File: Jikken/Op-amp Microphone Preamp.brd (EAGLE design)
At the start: 100 x 80 mm, 11 parts, among them IC1 AD822N

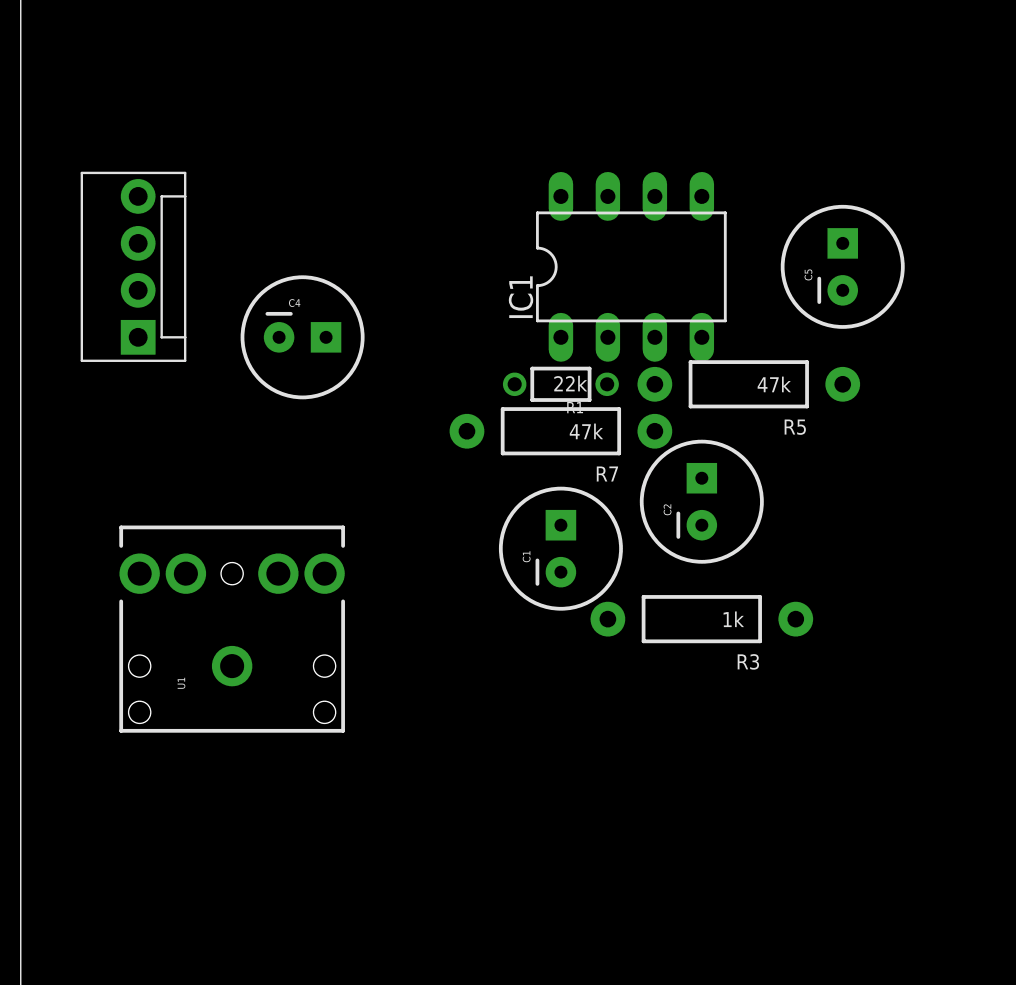
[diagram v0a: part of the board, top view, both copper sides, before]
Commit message: Preamp
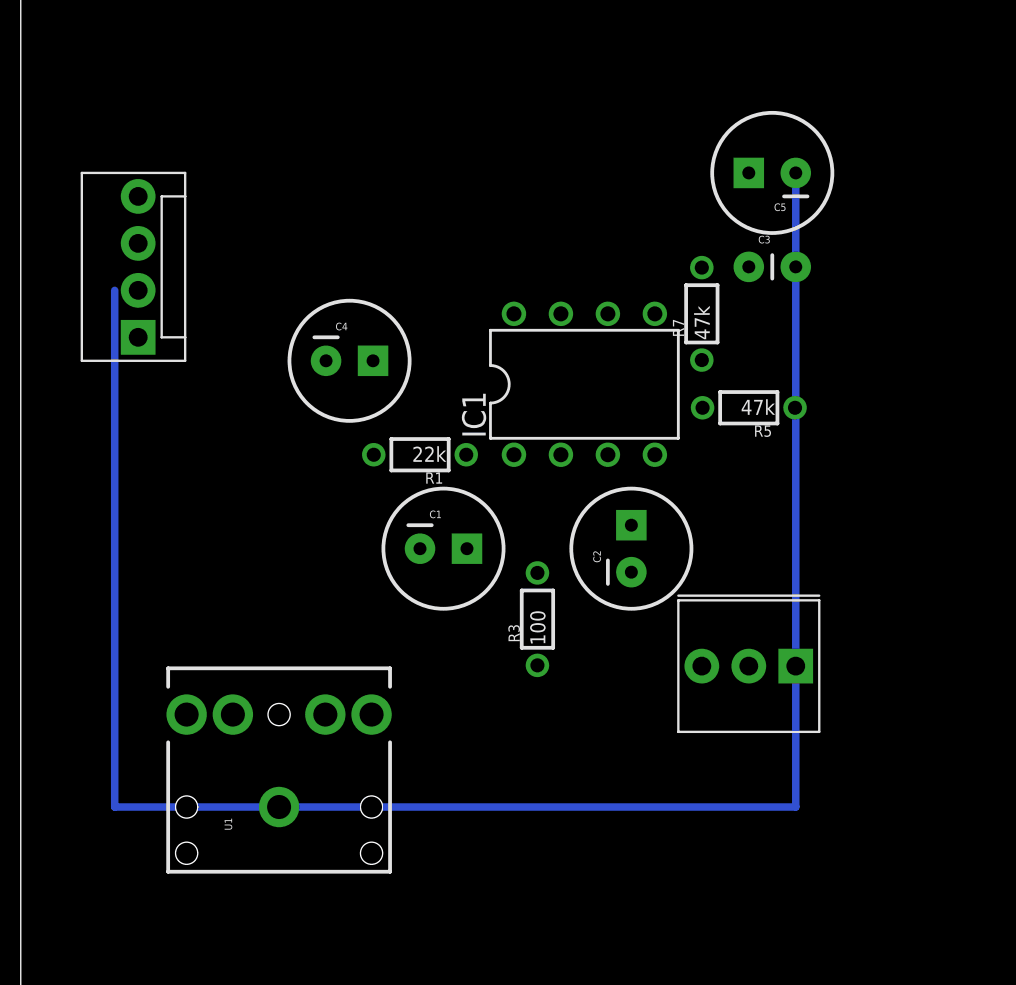
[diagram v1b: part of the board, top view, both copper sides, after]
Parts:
- added C3: 0.1uF, SparkFun:CAP-PTH-SMALL
- added TRIMPOT: 10k, My Library:3362U
- IC1: value AD822N -> LF356N; device analog-devices:DIL08 -> My Library:DIL08
- R3: value 1k -> 100; device SparkFun:AXIAL-0.4 -> SparkFun:1/6W-RES
- R5, R7: device SparkFun:AXIAL-0.4 -> SparkFun:1/6W-RES
- moved R7 9.92 mm to (36.8, 47.0), turned to 90 degrees
- moved R3 8.89 mm to (27.9, 30.5), turned to 90 degrees
- moved R1 8.52 mm to (21.6, 39.4)
- moved U1 8.03 mm to (14.0, 20.3)
- moved IC1 6.84 mm to (30.5, 43.2)
- moved C1 6.35 mm to (22.9, 34.3), turned to 0 degrees
- moved C5 6.35 mm to (40.6, 54.6), turned to 180 degrees
- moved C2 4.58 mm to (33.0, 34.3)
- moved C4 2.84 mm to (17.8, 44.5)
- moved R5 1.27 mm to (39.4, 41.9)
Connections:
- new net N$4: R3.1, TRIMPOT.P$2, TRIMPOT.P$3
- net GND: now also C3.2, R5.1, TRIMPOT.P$1; no longer R3.P$1, R5.P$1
- net N$2: now also R3.2; no longer R3.P$2
- net N$3: now also IC1.6; no longer IC1.1
- net N$6: now also R5.2, R7.1; no longer R5.P$2, R7.P$1
- net VCC: now also C3.1, IC1.7, R7.2; no longer IC1.8, R7.P$2
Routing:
- net GND: track 0.00 -> 99.1 mm
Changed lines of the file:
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@@
 </autorouter>
 <elements>
-<element name="IC1" library="analog-devices" package="DIL08" value="AD822N" x="33.02" y="49.53">
-<attribute name="OC_NEWARK" value="unknown" x="52.07" y="17.78" size="1.778" layer="27" display="off"/>
-<attribute name="MPN" value="" x="52.07" y="17.78" size="1.778" layer="27" display="off"/>
-<attribute name="MF" value="" x="52.07" y="17.78" size="1.778" layer="27" display="off"/>
-<attribute name="OC_FARNELL" value="1438581" x="52.07" y="17.78" size="1.778" layer="27" display="off"/>
-</element>
-<element name="R1" library="My Library" package="1/6W-RES" value="22k" x="29.21" y="43.18" rot="R180"/>
-<element name="R3" library="SparkFun" package="AXIAL-0.4" value="1k" x="36.83" y="30.48" rot="R180"/>
-<element name="C1" library="SparkFun" package="CPOL-RADIAL-100UF-25V" value="10u" x="29.21" y="34.29" rot="R90"/>
-<element name="R5" library="SparkFun" package="AXIAL-0.4" value="47k" x="39.37" y="43.18" rot="R180"/>
-<element name="U1" library="SparkFun" package="AUDIO-JACK" value="" x="11.43" y="27.94" rot="R90"/>
-<element name="R7" library="SparkFun" package="AXIAL-0.4" value="47k" x="29.21" y="40.64" rot="R180"/>
-<element name="C5" library="SparkFun" package="CPOL-RADIAL-100UF-25V" value="100u" x="44.45" y="49.53" rot="R90"/>
+<element name="R1" library="My Library" package="1/6W-RES" value="22k" x="21.59" y="39.37" rot="R180"/>
+<element name="R3" library="SparkFun" package="1/6W-RES" value="100" x="27.94" y="30.48" rot="R90"/>
+<element name="C1" library="SparkFun" package="CPOL-RADIAL-100UF-25V" value="10u" x="22.86" y="34.29"/>
+<element name="R5" library="SparkFun" package="1/6W-RES" value="47k" x="39.37" y="41.91" rot="R180"/>
+<element name="U1" library="SparkFun" package="AUDIO-JACK" value="" x="13.97" y="20.32" rot="R90"/>
+<element name="R7" library="SparkFun" package="1/6W-RES" value="47k" x="36.83" y="46.99" rot="R90"/>
+<element name="C5" library="SparkFun" package="CPOL-RADIAL-100UF-25V" value="100u" x="40.64" y="54.61" rot="R180"/>
 <element name="JP2" library="SparkFun" package="MOLEX-1X4" value="" x="6.35" y="45.72" rot="R90"/>
-<element name="C4" library="SparkFun" package="CPOL-RADIAL-100UF-25V" value="10u" x="15.24" y="45.72"/>
-<element name="C2" library="SparkFun" package="CPOL-RADIAL-100UF-25V" value="10u" x="36.83" y="36.83" rot="R90"/>
+<element name="C4" library="SparkFun" package="CPOL-RADIAL-100UF-25V" value="10u" x="17.78" y="44.45"/>
+<element name="C2" library="SparkFun" package="CPOL-RADIAL-100UF-25V" value="10u" x="33.02" y="34.29" rot="R90"/>
+<element name="IC1" library="My Library" package="DIL08" value="LF356N" x="30.48" y="43.18"/>
+<element name="TRIMPOT" library="My Library" package="3362U" value="10k" x="41.91" y="30.48" rot="R180"/>
+<element name="C3" library="SparkFun" package="CAP-PTH-SMALL" value="0.1uF" x="39.37" y="49.53"/>
 </elements>
 <signals>
 <signal name="N$3">
 <contactref element="R1" pad="2"/>
-<contactref element="IC1" pad="1"/>
 <contactref element="C4" pad="1"/>
-<wire x1="26.71" y1="43.18" x2="29.21" y2="45.72" width="0" layer="19" extent="1-1"/>
-<wire x1="16.51" y1="45.72" x2="29.21" y2="45.72" width="0" layer="19" extent="1-1"/>
+<contactref element="IC1" pad="6"/>
+<wire x1="19.05" y1="44.45" x2="31.75" y2="46.99" width="0" layer="19" extent="1-1"/>
+<wire x1="19.09" y1="39.37" x2="19.05" y2="44.45" width="0" layer="19" extent="1-1"/>
 </signal>
 <signal name="N$5">
-<contactref element="IC1" pad="2"/>
 <contactref element="C1" pad="1"/>
 <contactref element="R1" pad="1"/>
-<wire x1="31.71" y1="43.18" x2="31.75" y2="45.72" width="0" layer="19" extent="1-1"/>
-<wire x1="29.21" y1="35.56" x2="31.71" y2="43.18" width="0" layer="19" extent="1-1"/>
+<contactref element="IC1" pad="2"/>
+<wire x1="24.13" y1="34.29" x2="24.09" y2="39.37" width="0" layer="19" extent="1-1"/>
+<wire x1="29.21" y1="39.37" x2="24.13" y2="34.29" width="0" layer="19" extent="1-1"/>
 </signal>
 <signal name="N$2">
-<contactref element="R3" pad="P$2"/>
+<contactref element="R3" pad="2"/>
 <contactref element="C1" pad="2"/>
-<wire x1="29.21" y1="33.02" x2="31.75" y2="30.48" width="0" layer="19" extent="1-1"/>
+<wire x1="21.59" y1="34.29" x2="27.94" y2="32.98" width="0" layer="19" extent="1-1"/>
 </signal>
 <signal name="GND">
+<contactref element="C5" pad="2"/>
+<contactref element="JP2" pad="2"/>
 <contactref element="IC1" pad="4"/>
-<contactref element="C5" pad="2"/>
-<contactref element="R5" pad="P$1"/>
+<contactref element="R5" pad="1"/>
 <contactref element="U1" pad="SLEEVE"/>
-<contactref element="JP2" pad="2"/>
-<contactref element="R3" pad="P$1"/>
-<wire x1="44.45" y1="43.18" x2="44.45" y2="48.26" width="0" layer="19" extent="1-1"/>
-<wire x1="36.83" y1="45.72" x2="44.45" y2="48.26" width="0" layer="19" extent="1-1"/>
-<wire x1="41.91" y1="30.48" x2="44.45" y2="43.18" width="0" layer="19" extent="1-1"/>
-<wire x1="6.35" y1="48.26" x2="36.83" y2="45.72" width="0" layer="19" extent="1-1"/>
-<wire x1="11.43" y1="27.94" x2="6.35" y2="48.26" width="0" layer="19" extent="1-1"/>
+<contactref element="TRIMPOT" pad="P$1"/>
+<contactref element="C3" pad="2"/>
+<wire x1="41.91" y1="54.61" x2="41.91" y2="20.32" width="0.4064" layer="16"/>
+<wire x1="41.91" y1="20.32" x2="5.08" y2="20.32" width="0.4064" layer="16"/>
+<wire x1="5.08" y1="20.32" x2="5.08" y2="48.26" width="0.4064" layer="16"/>
+<wire x1="41.91" y1="54.61" x2="41.91" y2="49.53" width="0" layer="19" extent="1-1"/>
+<wire x1="6.35" y1="48.26" x2="5.08" y2="48.26" width="0" layer="19" extent="16-16"/>
+<wire x1="41.87" y1="41.91" x2="41.91" y2="49.53" width="0" layer="19" extent="1-1"/>
+<wire x1="41.91" y1="27.94" x2="41.91" y2="20.32" width="0" layer="19" extent="16-16"/>
+<wire x1="34.29" y1="39.37" x2="41.87" y2="41.91" width="0" layer="19" extent="1-1"/>
+<wire x1="13.97" y1="20.32" x2="5.08" y2="20.32" width="0" layer="19" extent="16-16"/>
 </signal>
 <signal name="N$6">
-<contactref element="R5" pad="P$2"/>
-<contactref element="R7" pad="P$1"/>
+<contactref element="R5" pad="2"/>
+<contactref element="R7" pad="1"/>
+<contactref element="C2" pad="1"/>
 <contactref element="IC1" pad="3"/>
-<contactref element="C2" pad="1"/>
-<wire x1="34.29" y1="40.64" x2="34.29" y2="45.72" width="0" layer="19" extent="1-1"/>
-<wire x1="34.29" y1="40.64" x2="34.29" y2="40.64" width="0" layer="19" extent="1-1"/>
-<wire x1="36.83" y1="38.1" x2="34.29" y2="40.64" width="0" layer="19" extent="1-1"/>
+<wire x1="36.87" y1="41.91" x2="36.83" y2="44.49" width="0" layer="19" extent="1-1"/>
+<wire x1="31.75" y1="39.37" x2="36.87" y2="41.91" width="0" layer="19" extent="1-1"/>
+<wire x1="33.02" y1="35.56" x2="31.75" y2="39.37" width="0" layer="19" extent="1-1"/>
 </signal>
 <signal name="VCC">
-<contactref element="IC1" pad="8"/>
 <contactref element="JP2" pad="3"/>
-<contactref element="R7" pad="P$2"/>
+<contactref element="R7" pad="2"/>
 <contactref element="C5" pad="1"/>
-<wire x1="29.21" y1="53.34" x2="44.45" y2="50.8" width="0" layer="19" extent="1-1"/>
-<wire x1="24.13" y1="40.64" x2="29.21" y2="53.34" width="0" layer="19" extent="1-1"/>
-<wire x1="6.35" y1="50.8" x2="24.13" y2="40.64" width="0" layer="19" extent="1-1"/>
+<contactref element="IC1" pad="7"/>
+<contactref element="C3" pad="1"/>
+<wire x1="39.37" y1="49.53" x2="39.37" y2="54.61" width="0" layer="19" extent="1-1"/>
+<wire x1="36.83" y1="49.49" x2="39.37" y2="49.53" width="0" layer="19" extent="1-1"/>
+<wire x1="29.21" y1="46.99" x2="36.83" y2="49.49" width="0" layer="19" extent="1-1"/>
+<wire x1="6.35" y1="50.8" x2="29.21" y2="46.99" width="0" layer="19" extent="1-1"/>
 </signal>
 <signal name="N$13">
 <contactref element="C4" pad="2"/>
 <contactref element="JP2" pad="1"/>
-<wire x1="6.35" y1="45.72" x2="13.97" y2="45.72" width="0" layer="19" extent="1-1"/>
+<wire x1="6.35" y1="45.72" x2="16.51" y2="44.45" width="0" layer="19" extent="1-1"/>
 </signal>
 <signal name="N$8">
 <contactref element="C2" pad="2"/>
 <contactref element="U1" pad="TIP"/>
-<wire x1="16.43" y1="32.94" x2="36.83" y2="35.56" width="0" layer="19" extent="1-1"/>
+<wire x1="18.97" y1="25.32" x2="33.02" y2="33.02" width="0" layer="19" extent="1-1"/>
 </signal>
 <signal name="N$9">
 <contactref element="U1" pad="RING"/>
 </signal>
+<signal name="N$4">
+<contactref element="R3" pad="1"/>
+<contactref element="TRIMPOT" pad="P$2"/>
+<contactref element="TRIMPOT" pad="P$3"/>
+<wire x1="36.83" y1="27.94" x2="27.94" y2="27.98" width="0" layer="19" extent="1-1"/>
+<wire x1="39.37" y1="27.94" x2="36.83" y2="27.94" width="0" layer="19" extent="1-1"/>
+</signal>
 </signals>
